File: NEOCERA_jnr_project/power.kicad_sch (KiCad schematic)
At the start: 26 parts, among them J1 USB_B, J3 770967-2, J4 770967-2, U10 LM7805_TO220, U11 LD39150DT33, U8 FT231XS, U9 HCPL-2630

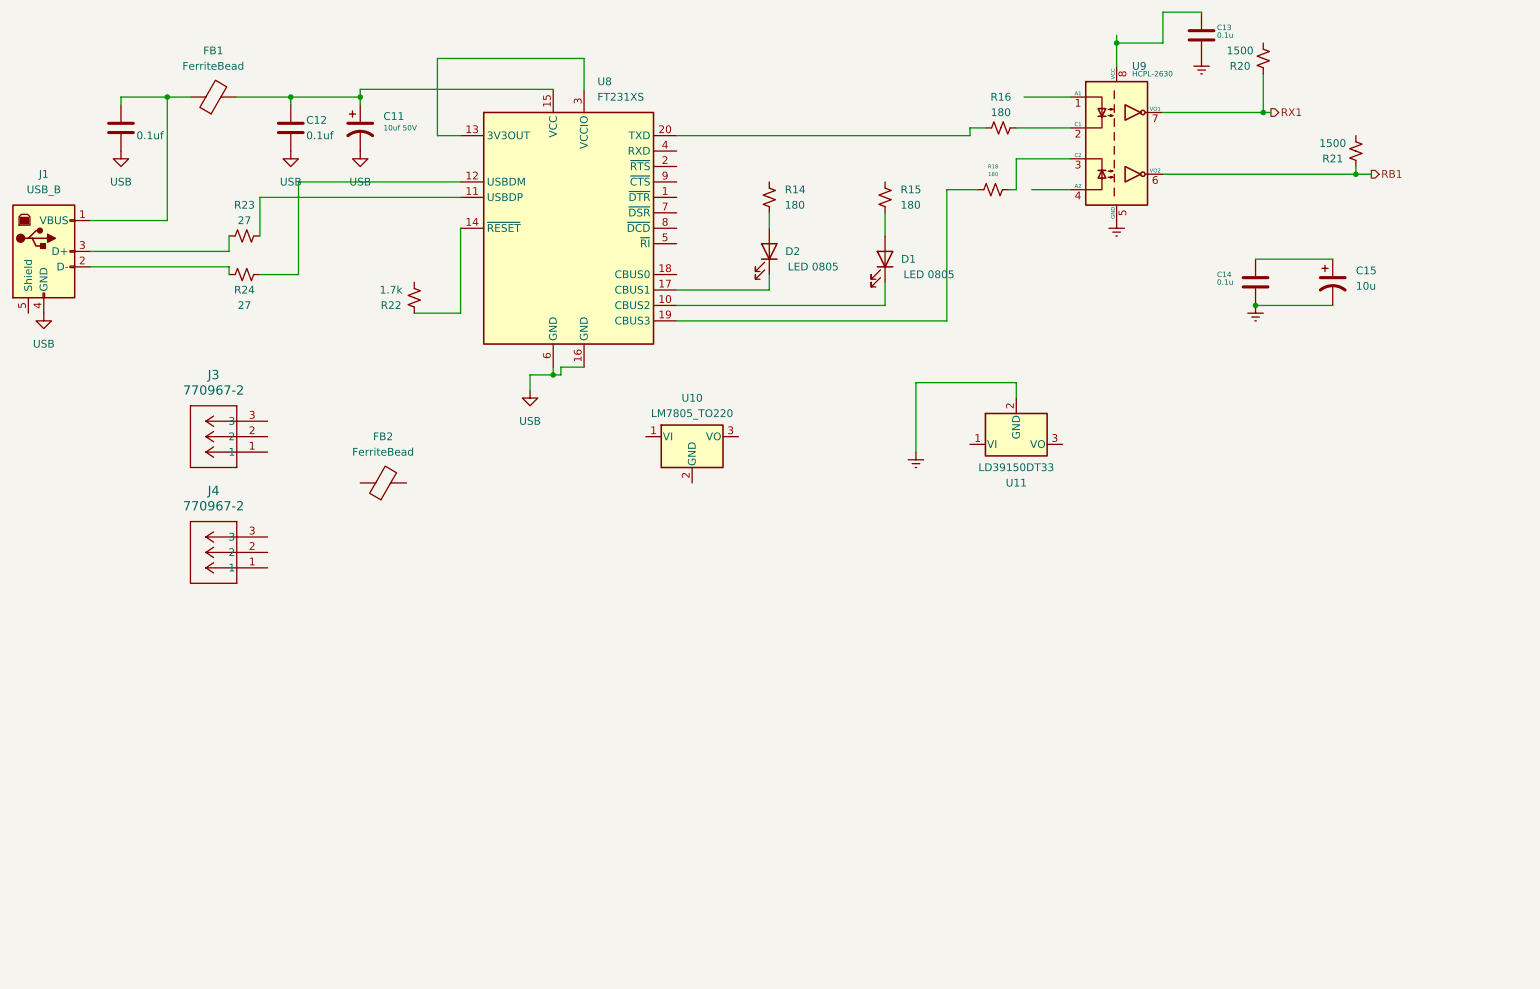
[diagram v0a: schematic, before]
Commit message: Update power.kicad_sch
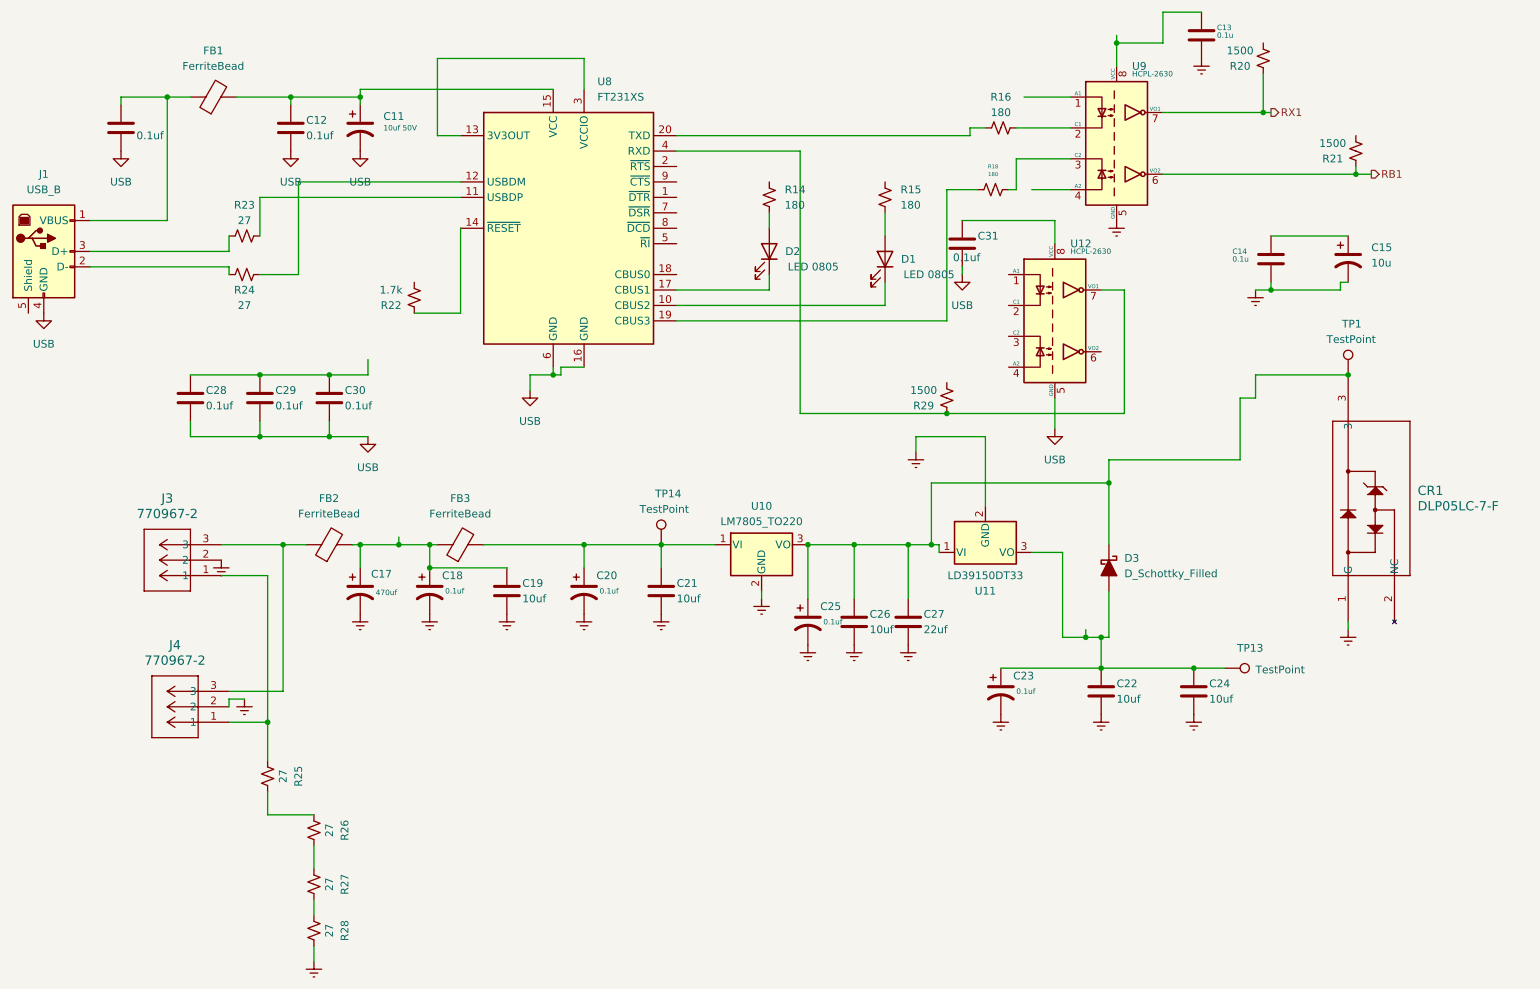
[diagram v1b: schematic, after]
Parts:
- added C17: 470uf, Capacitor_SMD:C_0603_1608Metric_Pad1.08x0.95mm_HandSolder, symbol Device:C_Polarized_US
- added C18, C20, C23, C25: 0.1uf, Capacitor_SMD:C_0603_1608Metric_Pad1.08x0.95mm_HandSolder, symbol Device:C_Polarized_US
- added C19, C21, C22, C24, C26: 10uf, Capacitor_SMD:C_0603_1608Metric_Pad1.08x0.95mm_HandSolder, symbol Device:C
- added C27: 22uf, Capacitor_SMD:C_0603_1608Metric_Pad1.08x0.95mm_HandSolder, symbol Device:C
- added C28, C29, C30, C31: 0.1uf, Capacitor_SMD:C_0603_1608Metric_Pad1.08x0.95mm_HandSolder, symbol Device:C
- added CR1: DLP05LC-7-F, SOT23_DLP05LC_DIO, symbol DLP05LC:DLP05LC-7-F
- added D3: D_Schottky_Filled, Diode_SMD:D_2114_3652Metric, symbol Device:D_Schottky_Filled
- added FB3: FerriteBead, Ferrite_THT:LairdTech_28C0236-0JW-10, symbol Device:FerriteBead
- added R25, R26, R27, R28: 27, Resistor_SMD:R_1206_3216Metric, symbol Device:R_Small_US
- added R29: 1500, Resistor_SMD:R_1206_3216Metric, symbol Device:R_Small_US
- added TP1, TP13, TP14: TestPoint, TestPoint:TestPoint_Loop_D2.50mm_Drill1.0mm, symbol Connector:TestPoint
- added U12: HCPL-2630, Package_DIP:DIP-8_W7.62mm, symbol Isolator:HCPL-2630
- C11, C12, C13, C14, C15, C16: footprint (none) -> Capacitor_SMD:C_0603_1608Metric_Pad1.08x0.95mm_HandSolder
- FB1, FB2: footprint (none) -> Ferrite_THT:LairdTech_28C0236-0JW-10
- J1: footprint (none) -> Connector_USB:USB_B_OST_USB-B1HSxx_Horizontal
- R14, R15, R16, R18, R20, R21, R22, R23, R24: footprint (none) -> Resistor_SMD:R_1206_3216Metric
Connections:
- net Earth: now also J3.2, J4.2, U10.2 (GND), C17.2, C18.2, C19.2, C20.2, C21.2, C22.2, C23.2, C24.2, C25.2, C26.2, C27.2, CR1.1 (G), R28.1
- net USB: now also C28.2, C29.2, C30.2, C31.2, U12.5 (GND)
- net at J4.1: now also J3.1, R25.2
- net at J4.3: now also FB2.1, J3.3
- net at U11.1 (VI): now also U10.3 (VO), C25.1, C26.1, C27.1, CR1.3, D3.1 (K), TP1.1
- net at U11.3 (VO): now also C22.1, C23.1, C24.1, D3.2 (A), TP13.1
- net at FB2.2: now also C17.1, C18.1, C19.1, FB3.1
- net at U10.1 (VI): now also C20.1, C21.1, FB3.2, TP14.1
- net at U8.4 (RXD): now also R29.1, U12.7 (VO1)
- new net: C28.1, C29.1, C30.1
- new net: C31.1, U12.8 (VCC)
- new net: R27.1, R28.2
- new net: R26.1, R27.2
- new net: R25.1, R26.2
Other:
- moved on the sheet: C14, C15, FB2, J3, J4, U10, U11
